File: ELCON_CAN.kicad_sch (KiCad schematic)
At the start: 9 parts, among them IC3 TCAN3413DR

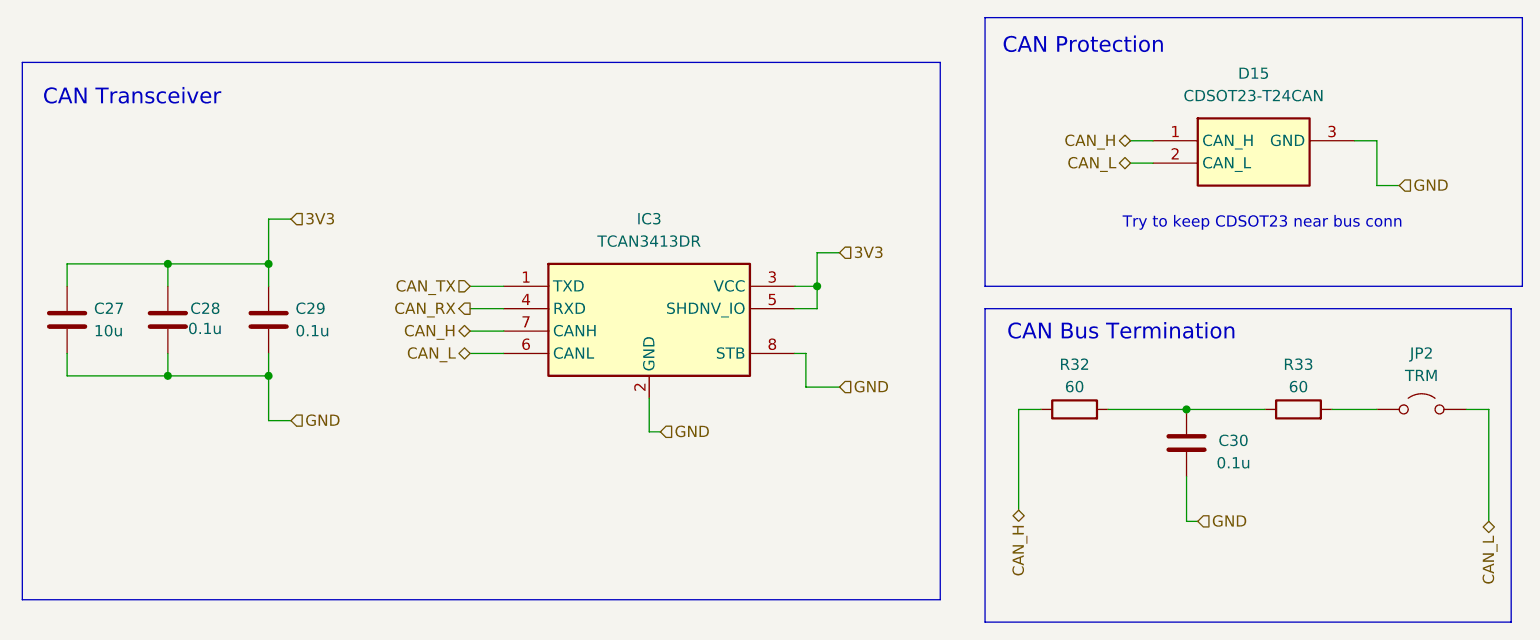
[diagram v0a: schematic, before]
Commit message: shoupu review done
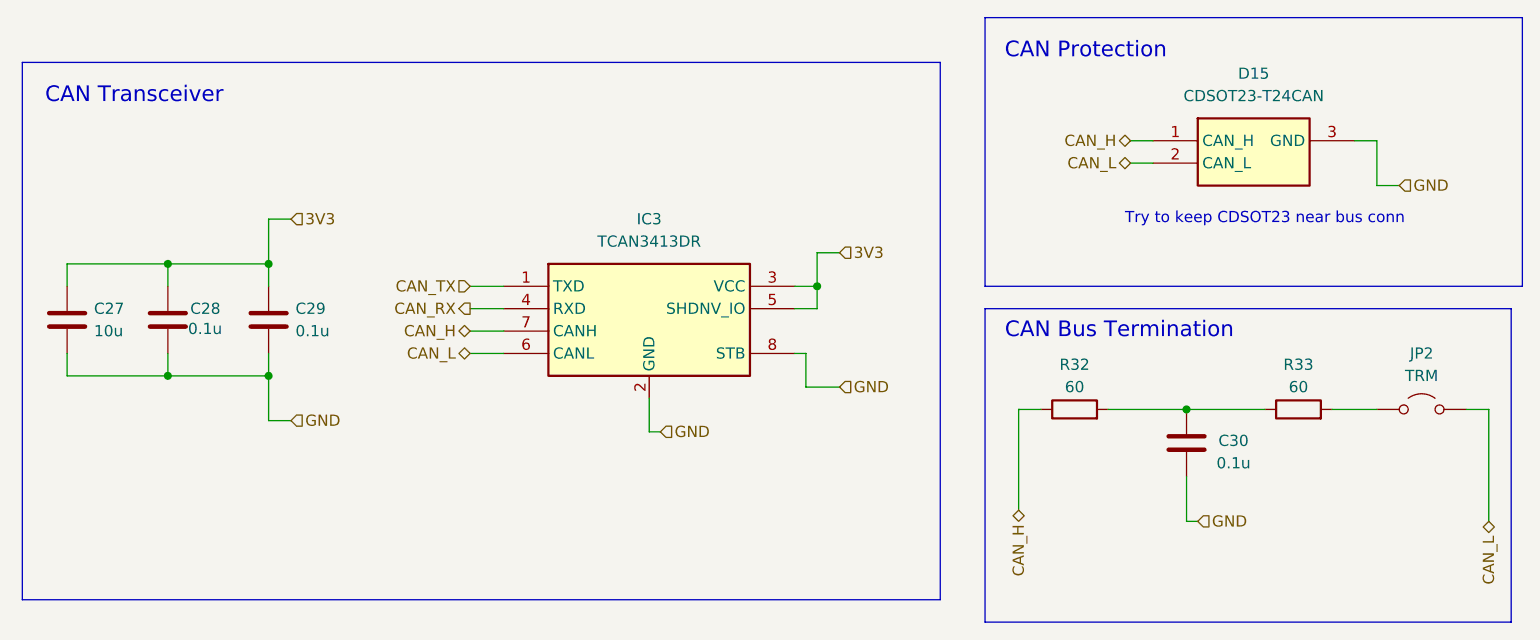
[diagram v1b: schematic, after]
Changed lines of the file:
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@@
 	(text "CAN Transceiver\n"
 		(exclude_from_sim no)
-		(at 81.026 65.024 0)
+		(at 81.28 64.77 0)
 		(effects
 			(font
@@
 	(text "Try to keep CDSOT23 near bus conn"
 		(exclude_from_sim no)
-		(at 209.296 79.248 0)
+		(at 209.55 78.74 0)
 		(effects
 			(font
@@
 	(text "CAN Protection"
 		(exclude_from_sim no)
-		(at 188.976 59.182 0)
+		(at 189.23 59.69 0)
 		(effects
 			(font
@@
 	(text "CAN Bus Termination\n"
 		(exclude_from_sim no)
-		(at 193.294 91.694 0)
+		(at 193.04 91.44 0)
 		(effects
 			(font
@@
 		)
 	)
-	(group "CAN_Transceiver"
-		(lib_id "LHRS_Design_Blocks:CAN_Transceiver")
-		(members "02dc0498-fa0a-4af4-999d-cc09ce2f8eed" "03ac9165-2ea4-425b-a3a2-2a3ac86ba5ac"
-			"0aab3452-ca44-4153-98ab-a4260fdc2c76" "0fcf45b8-2eeb-4956-88e8-96a8f3be2fc2"
-			"11fc3897-418c-456a-8fd5-75858f7bdad9" "14f6a92d-e85d-4654-93c9-436d0a52c752"
-			"16805fa4-525f-4785-8211-5b63dd1de1ce" "16ba06cb-8cbf-4ba2-8961-aabeac5c19e1"
-			"18a7dca3-e6ee-4f48-9c9e-fc76fa664e75" "1c957308-eb52-4c84-9d6f-48ae590d99d5"
-			"257454c3-1cbb-49bf-ac29-55b2bfc39800" "269c1b14-22dd-4a9f-bc64-46d9c4d23a1e"
-			"281fa88c-8ae1-4054-a13f-0c13c1d01bee" "2e405b7a-06f0-48f6-9cb5-8f138f157a54"
-			"34e9e19a-645e-4817-a53b-11ea4ec15937" "35735da6-cd68-4170-b8db-e419be0a1130"
-			"370fd011-4489-4130-aa09-5d1b9e226549" "3b4100a3-bbf0-46c4-b8f7-040bd2249cf8"
-			"3f3478ae-d264-4a67-9c59-7de031940324" "418918ed-79a5-4844-a068-77984ff1998e"
-			"43f094ec-461c-47c8-8122-1579148b6876" "45287061-c17c-4466-8f07-f5b0dbdf1e9e"
-			"457dd79d-04ce-4791-9e74-72678c3e65d8" "46a5c127-3bac-418c-9a75-8e883898b804"
-			"48b6a63b-2433-49e2-af21-5e7116c95b39" "4988521a-bb8e-4fb6-9e79-ab3f0d7c608b"
-			"4ed1fe97-086c-4c08-b22d-2fb1ba74a4d8" "53fc980d-cf29-4e0c-92a6-a4c6e65a77b0"
-			"70dac787-f0ab-4692-8f06-9e8bac98967d" "7443ee25-b112-418a-a19e-16b199a8fe5b"
-			"7460588d-8899-4373-b50b-fb0610e09f09" "7484bcdc-1ddf-4a31-9ac2-deff0b8d2fc5"
-			"76db90f1-78d8-4e5d-9cce-f6cfc8c68aa6" "7da5c6ca-1f5e-4e0c-9ed1-f5b25519203e"
-			"7fbf7d87-9fc4-40ea-820f-437fbcd62764" "80bc5ad1-4fbc-4a16-aff6-a41b50d0d5ed"
-			"89eda2dc-1a3a-4862-9057-2a53d23dc041" "8bc6d0f8-90a9-4a3e-bd4c-4f1d37db40e4"
-			"8cc7381c-268a-4e89-868e-d70c2ee1b2cf" "8d41f674-d426-4441-aa5f-d30bc0e8d498"
-			"8df04a62-6241-4b31-a5a9-801f1c6fce5c" "8e0b5df4-2cb8-49e3-8752-25e60af29d36"
-			"917c37b0-a50f-41a8-b594-d9c0c3e21ae7" "91f995af-5ad6-4388-b5d2-2ba28b704c70"
-			"920219a8-99ce-41b7-b456-4157126609a6" "92d7acaa-73a4-4711-9c6e-9d6f8e4b6bdf"
-			"97b807a7-2a0f-4f78-9be9-1b8fd00655be" "a20ab9fc-69aa-4ee0-93d6-3059b329d369"
-			"a3b72bfe-2a6f-42d8-b935-ec83e721d0d8" "a9bf4fee-14de-4ca1-87dd-71b6c8614922"
-			"aa55e51e-ff1d-4754-99e3-0cbf4fe8be3f" "adda2c19-4d52-4a5f-bfa0-e29c5e28dc27"
-			"b3caedac-de22-46e7-9643-c5c9196010b4" "b8ab2e19-3037-4588-b198-c07c4e77bc05"
-			"bb14a602-1916-4238-a873-64ed2a18b066" "c47537e4-6cb2-42bd-9e36-f2fdbbd88467"
-			"c568e6ca-7f97-4122-a9d3-1ff49abf5acc" "c6b18540-3af2-482b-b230-c7c3e88c1c2b"
-			"c72b6064-24ff-42cf-85a2-5f319e80bac0" "c84a68a2-25c9-4949-9cd3-564dce7f418d"
-			"c8de0135-271c-4834-b458-949e66171a03" "d0cd01de-532c-4881-bbfa-68dada0141bd"
-			"d3dc1093-5927-44fd-b183-035a11ec5677" "d72421b8-96df-4d96-96de-366e757e0c7f"
-			"d7bbf058-1019-472a-b210-c9dc6eda02c8" "deaa5507-d4de-4c93-9ade-af6e02b24328"
-			"e3b93d3c-a2e0-469f-9761-2465843355a0" "e61835ce-d874-4c37-a616-6e7e018e402e"
-			"e95fa83f-96e3-4782-8016-c95c1e9ac089" "e9ec658b-ebce-4051-855c-5a456c917486"
-			"eb3c1286-6fe4-4dc7-afe3-b68d2675cf98" "ef028e55-728d-474b-8b10-caf293163e9f"
-			"f1342c2b-b829-43d4-8ac0-e31472078542" "f1545d5e-e8b8-4f5b-9625-3f5248400e82"
-			"f28cb6b3-08af-4a21-962e-c691a9e4d85a" "f525b581-e914-48f3-856d-b707a04117a7"
-			"f6b33fcd-5bfe-4b47-8ac1-5aada0c5cd35" "f905bbd5-25e3-4518-9a89-c3e959777327"
-			"f97194eb-8b04-459a-bd92-5670cfc15c32" "f98052f3-8ad3-423e-8537-c8cb59b58c1e"
-			"fe08bceb-d9f3-4168-a413-0146d6218e26"
-		)
-	)
